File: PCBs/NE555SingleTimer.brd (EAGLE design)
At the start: 24.2 x 19 mm, 7 parts, among them T1 2N3904

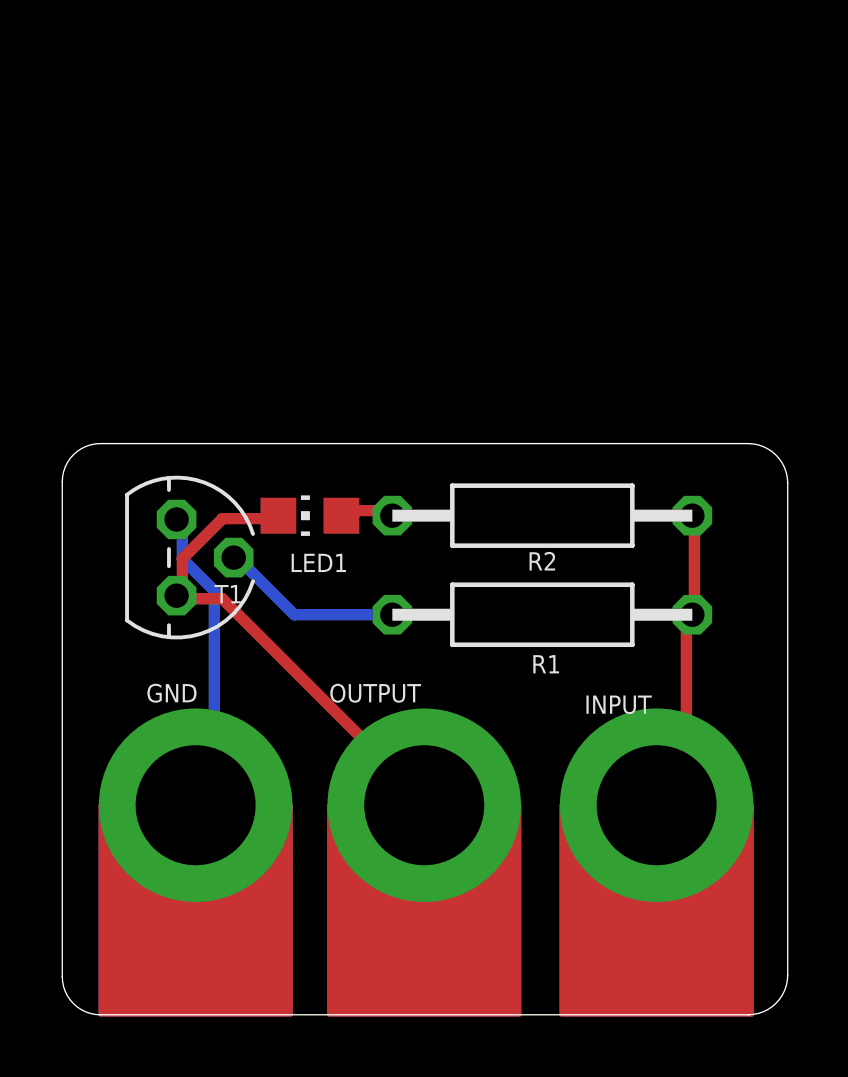
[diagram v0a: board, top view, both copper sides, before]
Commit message: Renamed files .
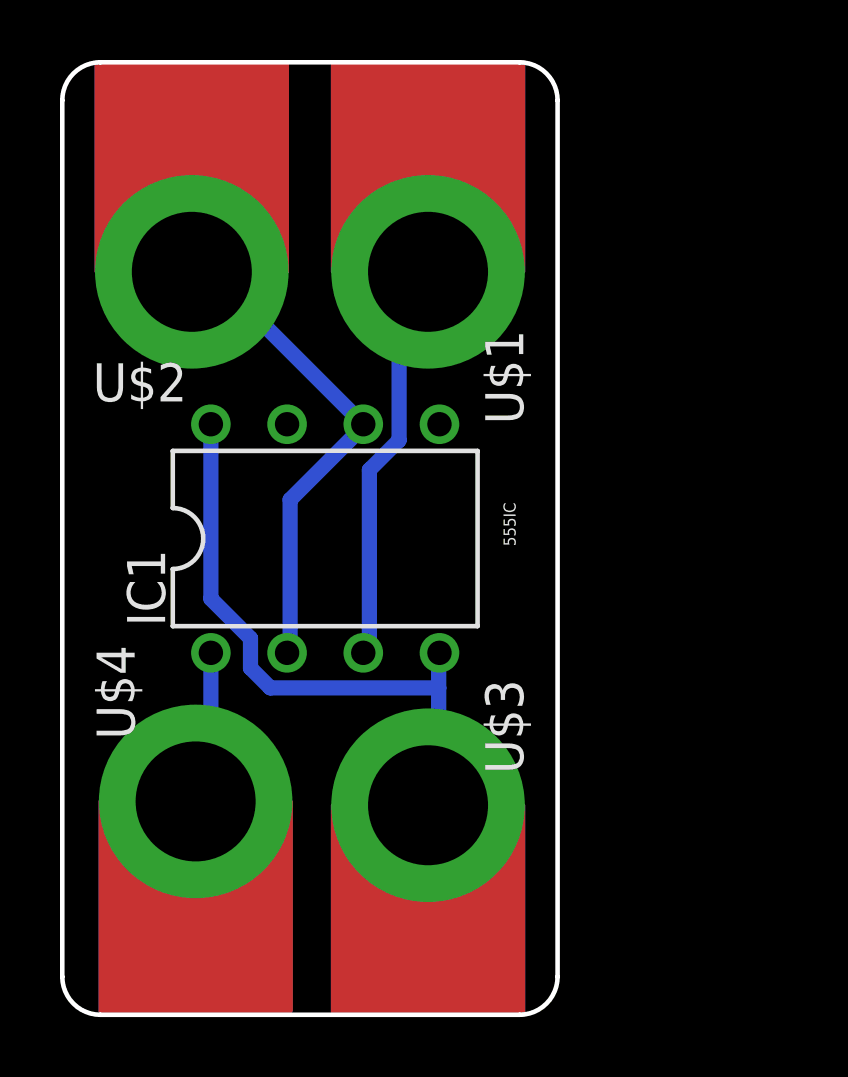
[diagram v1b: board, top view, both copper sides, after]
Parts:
- removed GND, INPUT, OUTPUT: MICROBIT_PAD, microbit:MICROBIT_PAD
- removed LED1: (no value), led:CHIP-LED0805
- removed R1, R2: (no value), we-rcl:R0207/10
- removed T1: 2N3904, transistor:TO92
- added IC1: LM555N, linear:DIL08
- added U$1, U$2, U$3, U$4: MICROBIT_PAD, microbit:MICROBIT_PAD
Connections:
- removed net N$3: R1.2, T1.2
- net 5V: now also IC1.4, IC1.8, U$3.PAD; no longer INPUT.PAD, R1.1, R2.2
- net GND: now also IC1.1, U$4.PAD; no longer GND.PAD, T1.3
- net N$1: now also IC1.3, U$1.PAD; no longer LED1.A, R2.1
- net N$2: now also IC1.2, IC1.6, U$2.PAD; no longer LED1.C, OUTPUT.PAD, T1.1
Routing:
- net N$1: track 1.95 -> 13.8 mm
- net 5V: track 10.3 -> 20.4 mm
- net N$3: track 6.06 -> 0.00 mm
- net GND: track 10.3 -> 5.17 mm
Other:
- board size 24.2 x 19 mm -> 16.5 x 31.8 mm
- board text added: "555IC"
